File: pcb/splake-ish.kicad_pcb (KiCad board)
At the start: 2 copper layers, 155.5 x 105 mm, 123 parts

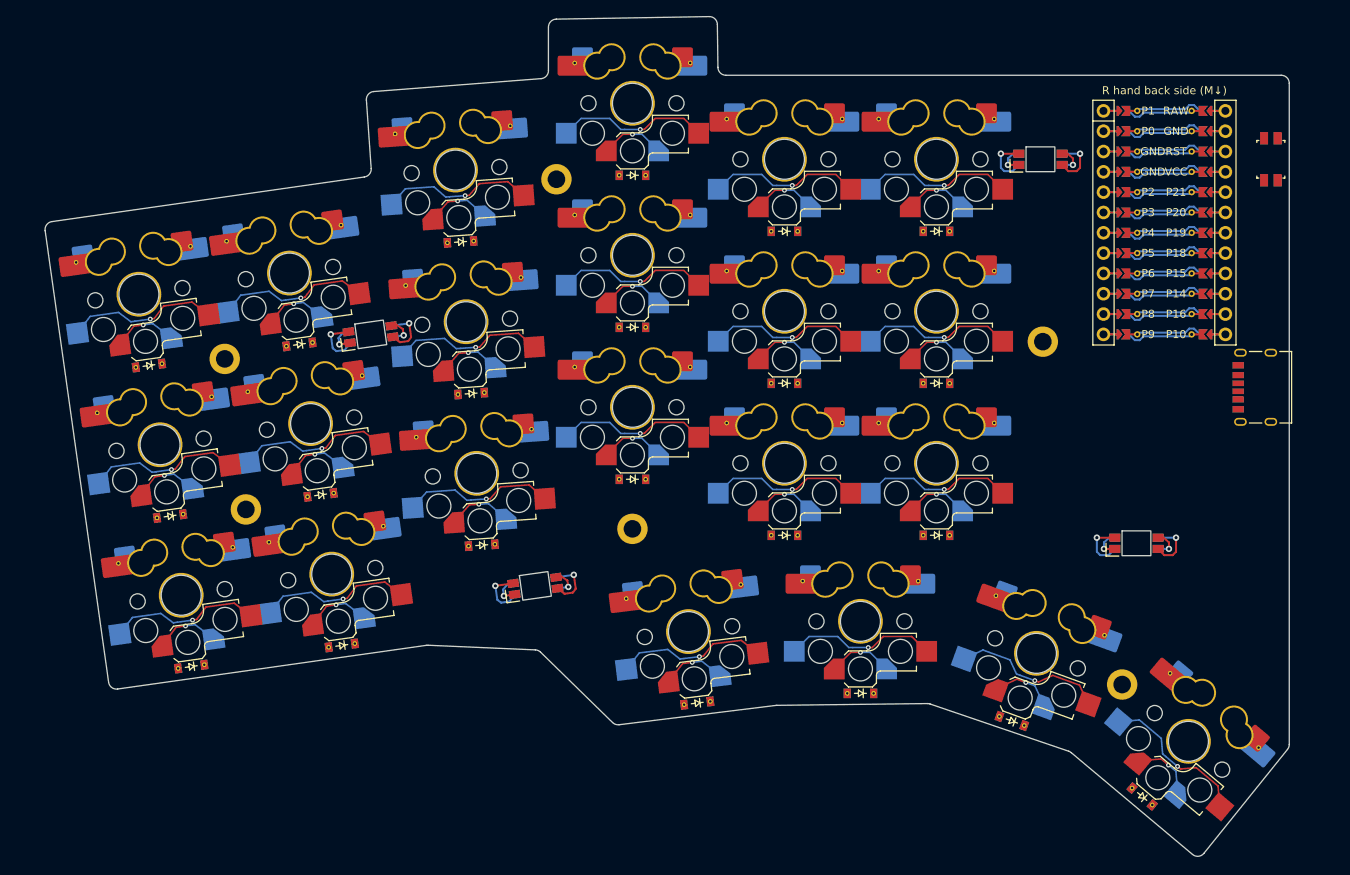
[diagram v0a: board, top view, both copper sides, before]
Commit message: final pcb V1
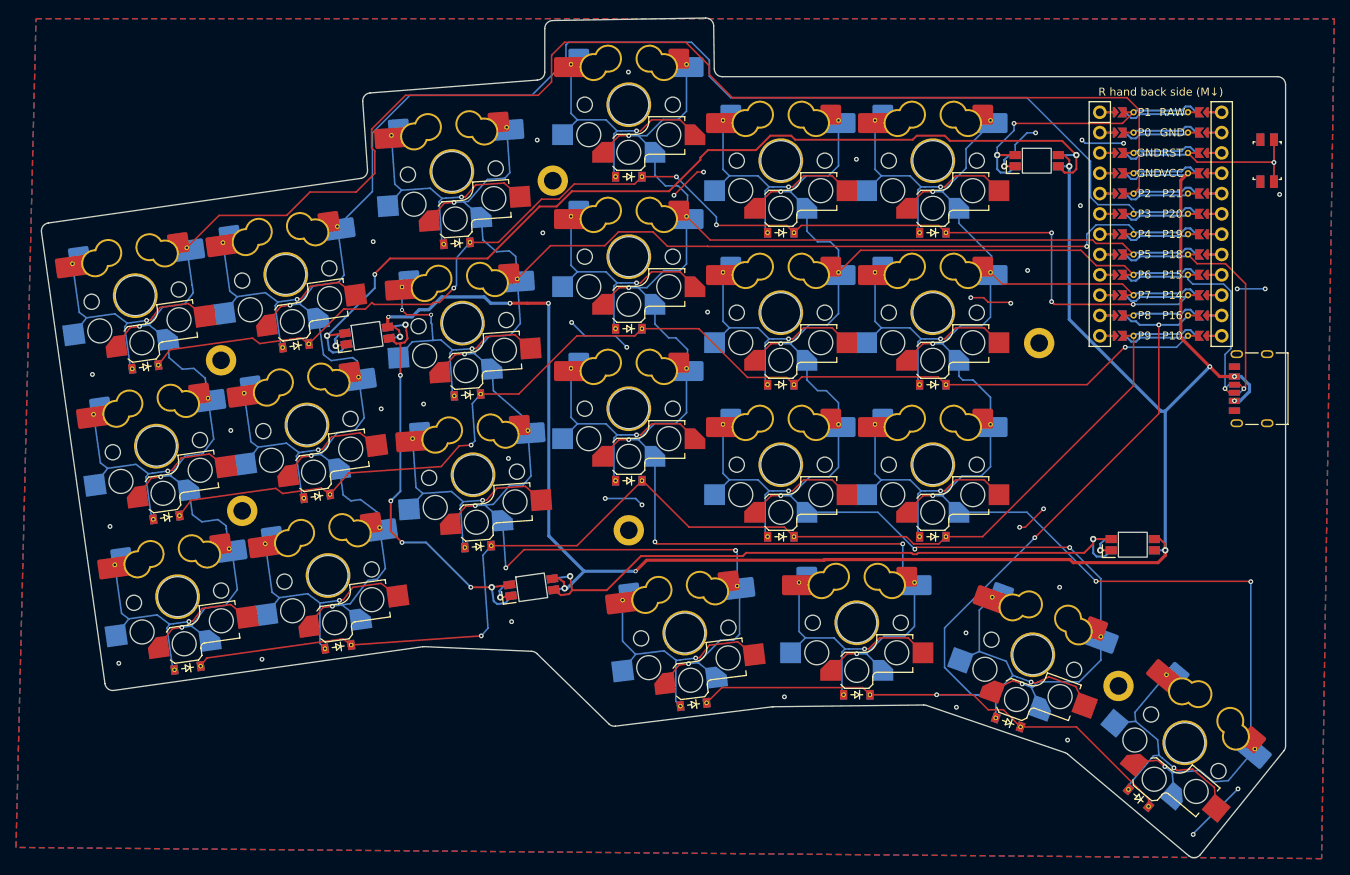
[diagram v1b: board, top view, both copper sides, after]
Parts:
- removed the REF** at (122.1, 146.0)
- removed the REF** at (179.2, 121.5)
- removed the REF** at (179.2, 102.5)
- removed the REF** at (179.2, 83.5)
- removed the REF** at (198.2, 128.5)
- removed the REF** at (198.2, 109.5)
- removed the REF** at (198.2, 90.5)
- removed the REF** at (217.2, 128.5)
- removed the REF** at (217.2, 109.5)
- removed the REF** at (217.2, 90.5)
- removed the REF** at (207.7, 148.2)
- removed the REF** at (119.5, 127.2)
- removed the REF** at (231.8, 150.1)
- removed the REF** at (253.6, 159.8)
- removed the REF** at (185.6, 150.4)
- removed the REF** at (136.4, 144.0)
- removed the REF** at (133.8, 125.2)
- removed the REF** at (131.2, 106.4)
- removed the REF** at (155.3, 141.4)
- removed the REF** at (152.6, 122.5)
- removed the REF** at (150.0, 103.7)
- removed the REF** at (173.8, 129.2)
- removed the REF** at (116.9, 108.4)
- removed the REF** at (172.5, 110.3)
- removed the REF** at (171.1, 91.3)
- removed the REF** at (193.6, 121.5)
- removed the REF** at (193.6, 102.5)
- removed the REF** at (193.6, 83.5)
- removed the REF** at (212.6, 128.5)
- removed the REF** at (212.6, 109.5)
- removed the REF** at (212.6, 90.5)
- removed the REF** at (231.6, 128.5)
- removed the REF** at (231.6, 109.5)
- removed the REF** at (141.0, 143.4)
- removed the REF** at (231.6, 90.5)
- removed the REF** at (222.1, 148.2)
- removed the REF** at (245.4, 155.0)
- removed the REF** at (264.7, 169.0)
- removed the REF** at (200.0, 148.7)
- removed the REF** at (138.3, 124.6)
- removed the REF** at (135.7, 105.7)
- removed the REF** at (159.4, 130.2)
- removed the REF** at (158.1, 111.3)
- removed the REF** at (156.7, 92.3)
- added REF**: VIA-0.6mm, VIA-0.6mm, F.Cu at (193.2, 83.6)
- added REF**: VIA-0.6mm, VIA-0.6mm, F.Cu at (173.3, 129.4)
- added REF**: VIA-0.6mm, VIA-0.6mm, F.Cu at (231.2, 109.6)
- added REF**: VIA-0.6mm, VIA-0.6mm, F.Cu at (199.5, 148.8)
- added REF**: VIA-0.6mm, VIA-0.6mm, F.Cu at (212.2, 90.6)
- added REF**: VIA-0.6mm, VIA-0.6mm, F.Cu at (245.0, 155.2)
- added REF**: VIA-0.6mm, VIA-0.6mm, F.Cu at (178.7, 121.6)
- added REF**: VIA-0.6mm, VIA-0.6mm, F.Cu at (172.0, 110.5)
- added REF**: VIA-0.6mm, VIA-0.6mm, F.Cu at (231.2, 90.6)
- added REF**: VIA-0.6mm, VIA-0.6mm, F.Cu at (178.7, 83.6)
- added REF**: VIA-0.6mm, VIA-0.6mm, F.Cu at (137.9, 124.7)
- added REF**: VIA-0.6mm, VIA-0.6mm, F.Cu at (231.2, 128.6)
- added REF**: VIA-0.6mm, VIA-0.6mm, F.Cu at (197.7, 128.6)
- added REF**: VIA-0.6mm, VIA-0.6mm, F.Cu at (197.7, 90.6)
- added REF**: VIA-0.6mm, VIA-0.6mm, F.Cu at (121.7, 146.2)
- added REF**: VIA-0.6mm, VIA-0.6mm, F.Cu at (212.2, 128.6)
- added REF**: VIA-0.6mm, VIA-0.6mm, F.Cu at (231.4, 150.2)
- added REF**: VIA-0.6mm, VIA-0.6mm, F.Cu at (185.2, 150.6)
- added REF**: VIA-0.6mm, VIA-0.6mm, F.Cu at (170.7, 91.5)
- added REF**: VIA-0.6mm, VIA-0.6mm, F.Cu at (119.0, 127.4)
- added REF**: VIA-0.6mm, VIA-0.6mm, F.Cu at (216.7, 90.6)
- added REF**: VIA-0.6mm, VIA-0.6mm, F.Cu at (253.2, 159.9)
- added REF**: VIA-0.6mm, VIA-0.6mm, F.Cu at (135.2, 105.9)
- added REF**: VIA-0.6mm, VIA-0.6mm, F.Cu at (264.2, 169.2)
- added REF**: VIA-0.6mm, VIA-0.6mm, F.Cu at (158.9, 130.4)
- added REF**: VIA-0.6mm, VIA-0.6mm, F.Cu at (133.3, 125.4)
- added REF**: VIA-0.6mm, VIA-0.6mm, F.Cu at (149.5, 103.9)
- added REF**: VIA-0.6mm, VIA-0.6mm, F.Cu at (157.6, 111.5)
- added REF**: VIA-0.6mm, VIA-0.6mm, F.Cu at (178.7, 102.6)
- added REF**: VIA-0.6mm, VIA-0.6mm, F.Cu at (193.2, 102.6)
- added REF**: VIA-0.6mm, VIA-0.6mm, F.Cu at (212.2, 109.6)
- added REF**: VIA-0.6mm, VIA-0.6mm, F.Cu at (136.0, 144.2)
- added REF**: VIA-0.6mm, VIA-0.6mm, F.Cu at (216.7, 109.6)
- added REF**: VIA-0.6mm, VIA-0.6mm, F.Cu at (197.7, 109.6)
- added REF**: VIA-0.6mm, VIA-0.6mm, F.Cu at (116.4, 108.6)
- added REF**: VIA-0.6mm, VIA-0.6mm, F.Cu at (156.3, 92.5)
- added REF**: VIA-0.6mm, VIA-0.6mm, F.Cu at (140.5, 143.6)
- added REF**: VIA-0.6mm, VIA-0.6mm, F.Cu at (207.2, 148.4)
- added REF**: VIA-0.6mm, VIA-0.6mm, F.Cu at (130.7, 106.6)
- added REF**: VIA-0.6mm, VIA-0.6mm, F.Cu at (152.2, 122.7)
- added REF**: VIA-0.6mm, VIA-0.6mm, F.Cu at (221.7, 148.4)
- added REF**: VIA-0.6mm, VIA-0.6mm, F.Cu at (154.8, 141.5)
- added REF**: VIA-0.6mm, VIA-0.6mm, F.Cu at (216.7, 128.6)
- added REF**: VIA-0.6mm, VIA-0.6mm, F.Cu at (193.2, 121.6)
- moved D19 0.49 mm to (214.4, 162.4)
- moved S19 0.49 mm to (214.4, 153.4)
- moved S41 0.49 mm to (214.4, 153.4)
- moved D20 0.49 mm to (233.4, 165.9)
- moved S13 0.49 mm to (204.9, 133.7)
- moved S35 0.49 mm to (204.9, 133.7)
- moved S30 0.49 mm to (165.2, 116.0)
- moved S8 0.49 mm to (165.2, 116.0)
- moved MCU1 0.49 mm to (252.4, 102.3)
- moved D14 0.49 mm to (204.9, 123.7)
- moved S1 0.49 mm to (129.5, 150.2)
- moved S23 0.49 mm to (129.5, 150.2)
- moved D10 0.49 mm to (185.9, 135.7)
- moved D4 0.49 mm to (149.6, 156.4)
- moved H3 0.49 mm to (176.4, 98.2)
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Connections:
- D22 pad 1: 1_r1 -> 1_r1_thumb2
- D22 pad 2: 1_r1 -> 1_r1_thumb2
- LED1 pad 2: rgb -> led2
- LED1 pad 4: rgb -> led1
- LED2 pad 2: rgb -> led3
- LED2 pad 4: rgb -> led2
- LED3 pad 2: rgb -> led1
- LED3 pad 4: rgb -> P1
- LED4 pad 2: rgb -> (no net)
- LED4 pad 4: rgb -> led3
- MCU1 pad 108: P18 -> CC2
- MCU1 pad 109: P15 -> CC1
- S22 pad 2: 1_r1 -> 1_r1_thumb2
- S44 pad : 1_r1 -> 1_r1_thumb2
- S44 pad 2: 1_r1 -> 1_r1_thumb2
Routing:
- net (no net): track 337.7 -> 0.00 mm
- net VCC: track 15.0 -> 256.9 mm, vias 4 -> 11
- net P2: track 24.8 -> 245.2 mm
- net P4: track 33.1 -> 238.3 mm, vias 4 -> 7
- net P3: track 24.8 -> 222.9 mm
- net P5: track 33.1 -> 221.8 mm, vias 4 -> 6
- net P6: track 33.1 -> 202.4 mm, vias 4 -> 6
- net P14: track 0.00 -> 164.6 mm, vias 0 -> 6
- net P7: track 33.1 -> 193.0 mm, vias 4 -> 6
- net P9: track 0.00 -> 159.3 mm, vias 0 -> 1
- net P10: track 0.00 -> 155.5 mm, vias 0 -> 2
- net P16: track 0.00 -> 138.2 mm, vias 0 -> 3
- net led1: track 0.00 -> 120.4 mm, vias 0 -> 3
- net led3: track 0.00 -> 81.8 mm, vias 0 -> 2
- net GND: track 15.0 -> 93.2 mm, vias 4 -> 44
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- added copper zone on B.Cu, net GND
- added copper zone on F.Cu, net GND
